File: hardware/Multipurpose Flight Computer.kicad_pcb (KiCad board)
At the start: 4 copper layers, 35.6 x 44.6 mm, 82 parts, among them J1 Screw_Terminal_01x02, J2 Conn_01x03, J3 Conn_01x03, SW1 TS-1088-AR02016, SW2 TS-1088-AR02016, U1 BQ25883RGER, U2 ICM-45686, U3 STM32F722RETx, U4 BMP580, U5 TPS63070RNMR, U6 LMR51430, X1 X322525MOB4SI, X2 Q13FC1350000400

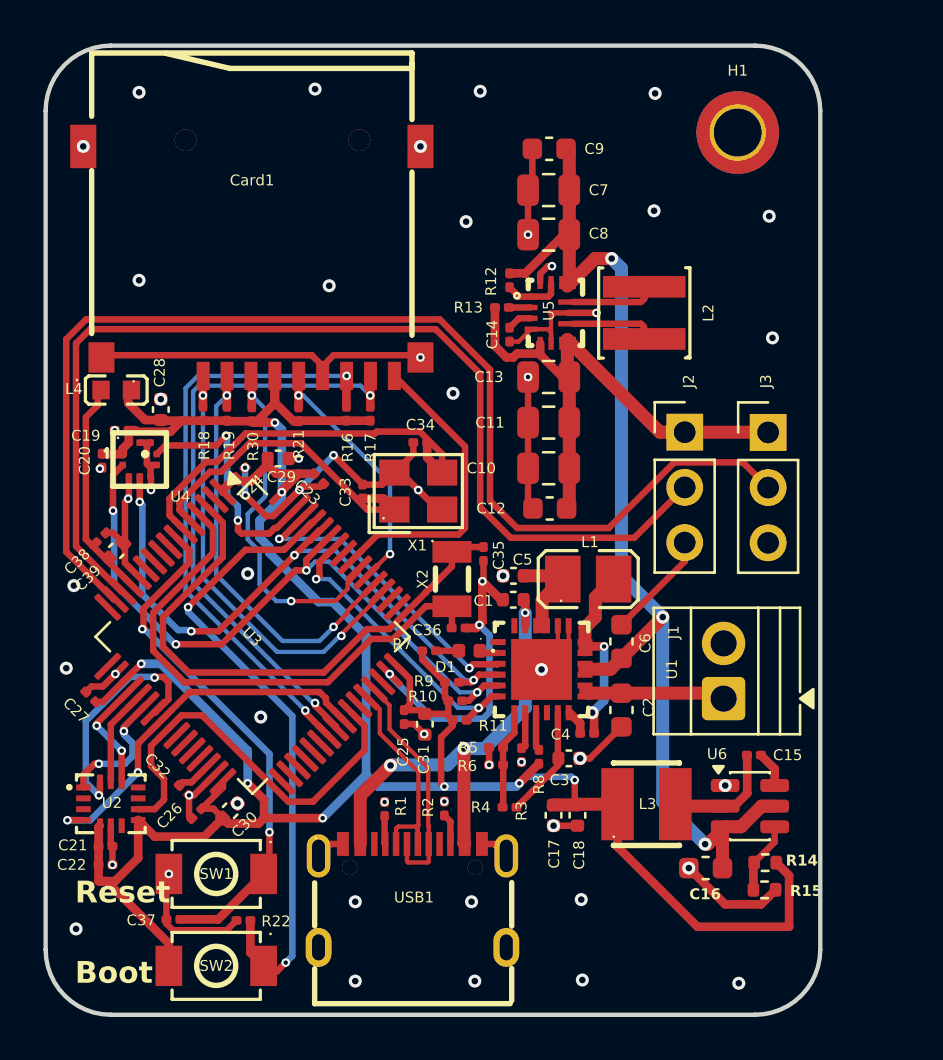
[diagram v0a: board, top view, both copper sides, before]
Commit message: minor edits
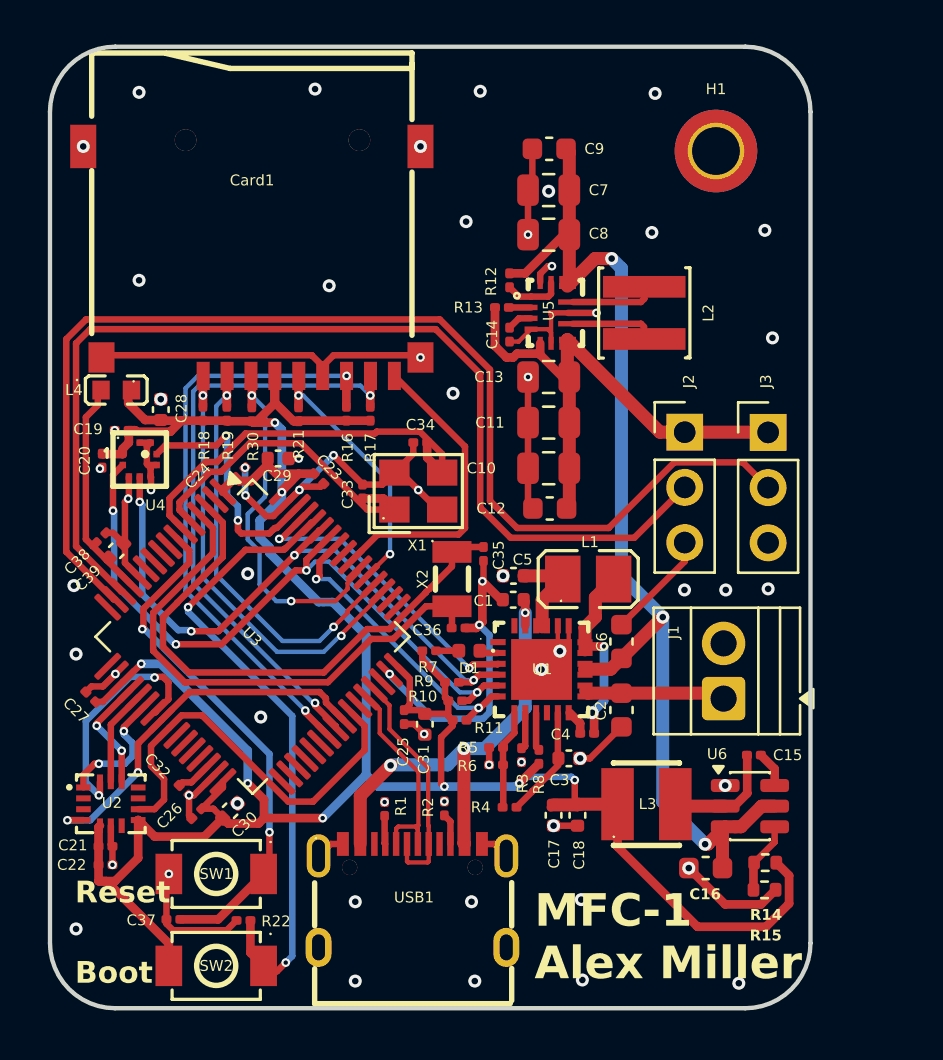
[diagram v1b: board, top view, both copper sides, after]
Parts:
- moved H1 1.31 mm to (155.7, 125.6)
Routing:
- net +3.3V: track 129.4 -> 128.8 mm
- net GND: vias 60 -> 65
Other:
- board size 35.6 x 44.6 mm -> 35 x 44.3 mm
- board text added: "MFC-1 Alex Miller"
